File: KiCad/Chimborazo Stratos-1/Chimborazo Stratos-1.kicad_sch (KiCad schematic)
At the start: 0 parts

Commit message: fixed long path errors and cleaned up libraries, finally I added the libs for the project it was REALLY HARD AND I DONT KNOW WHY :( but I managed to overcome the challenge
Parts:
- added U1: RP2040, Package_DFN_QFN:QFN-56-1EP_7x7mm_P0.4mm_EP3.2x3.2mm, symbol MCU_RaspberryPi:RP2040
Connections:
- new net: U1.1 (IOVDD), U1.10 (IOVDD), U1.22 (IOVDD), U1.33 (IOVDD), U1.42 (IOVDD), U1.49 (IOVDD)
- new net: U1.23 (DVDD), U1.50 (DVDD)
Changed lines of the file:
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@@
 	(generator_version "9.0")
 	(paper "A4")
+	(symbol
+		(lib_id "MCU_RaspberryPi:RP2040")
+		(at 140.97 80.01 0)
+		(unit 1)
+		(exclude_from_sim no)
+		(in_bom yes)
+		(on_board yes)
+		(dnp no)
+		(fields_autoplaced yes)
+		(property "Reference" "U1"
+			(at 143.1133 124.46 0)
+			(effects
+				(font
+					(size 1.27 1.27)
+				)
+				(justify left)
+			)
+		)
+		(property "Value" "RP2040"
+			(at 143.1133 127 0)
+			(effects
+				(font
+					(size 1.27 1.27)
+				)
+				(justify left)
+			)
+		)
+		(property "Footprint" "Package_DFN_QFN:QFN-56-1EP_7x7mm_P0.4mm_EP3.2x3.2mm"
+			(at 140.97 80.01 0)
+			(effects
+				(font
+					(size 1.27 1.27)
+				)
+				(hide yes)
+			)
+		)
+		(property "Datasheet" "https://datasheets.raspberrypi.com/rp2040/rp2040-datasheet.pdf"
+			(at 140.97 80.01 0)
+			(effects
+				(font
+					(size 1.27 1.27)
+				)
+				(hide yes)
+			)
+		)
+		(property "Description" "A microcontroller by Raspberry Pi"
+			(at 140.97 80.01 0)
+			(effects
+				(font
+					(size 1.27 1.27)
+				)
+				(hide yes)
+			)
+		)
+		(pin "13"
+		)
+		(pin "27"
+		)
+		(pin "20"
+		)
+		(pin "48"
+		)
+		(pin "46"
+		)
+		(pin "55"
+		)
+		(pin "34"
+		)
+		(pin "36"
+		)
+		(pin "38"
+		)
+		(pin "40"
+		)
+		(pin "19"
+		)
+		(pin "56"
+		)
+		(pin "15"
+		)
+		(pin "54"
+		)
+		(pin "10"
+		)
+		(pin "45"
+		)
+		(pin "53"
+		)
+		(pin "42"
+		)
+		(pin "26"
+		)
+		(pin "4"
+		)
+		(pin "47"
+		)
+		(pin "57"
+		)
+		(pin "5"
+		)
+		(pin "51"
+		)
+		(pin "43"
+		)
+		(pin "3"
+		)
+		(pin "33"
+		)
+		(pin "1"
+		)
+		(pin "50"
+		)
+		(pin "2"
+		)
+		(pin "6"
+		)
+		(pin "7"
+		)
+		(pin "9"
+		)
+		(pin "11"
+		)
+		(pin "21"
+		)
+		(pin "8"
+		)
+		(pin "12"
+		)
+		(pin "24"
+		)
+		(pin "25"
+		)
+		(pin "23"
+		)
+		(pin "52"
+		)
+		(pin "49"
+		)
+		(pin "44"
+		)
+		(pin "14"
+		)
+		(pin "22"
+		)
+		(pin "16"
+		)
+		(pin "17"
+		)
+		(pin "18"
+		)
+		(pin "28"
+		)
+		(pin "29"
+		)
+		(pin "30"
+		)
+		(pin "31"
+		)
+		(pin "32"
+		)
+		(pin "35"
+		)
+		(pin "37"
+		)
+		(pin "39"
+		)
+		(pin "41"
+		)
+		(instances
+			(project ""
+				(path "/693bdab5-43ca-4fa8-b8fd-c6e41a7a7cc1"
+					(reference "U1")
+					(unit 1)
+				)
+			)
+		)
+	)
 	(sheet_instances
 		(path "/"

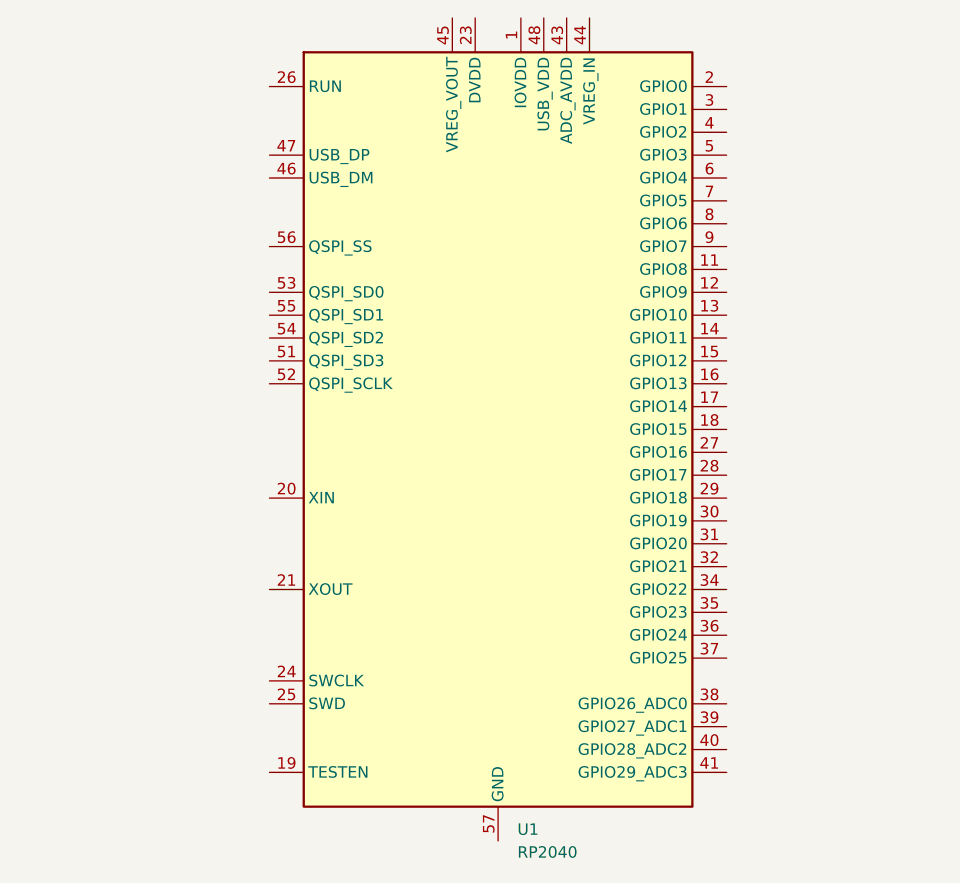
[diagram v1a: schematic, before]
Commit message: Schematic prototype done
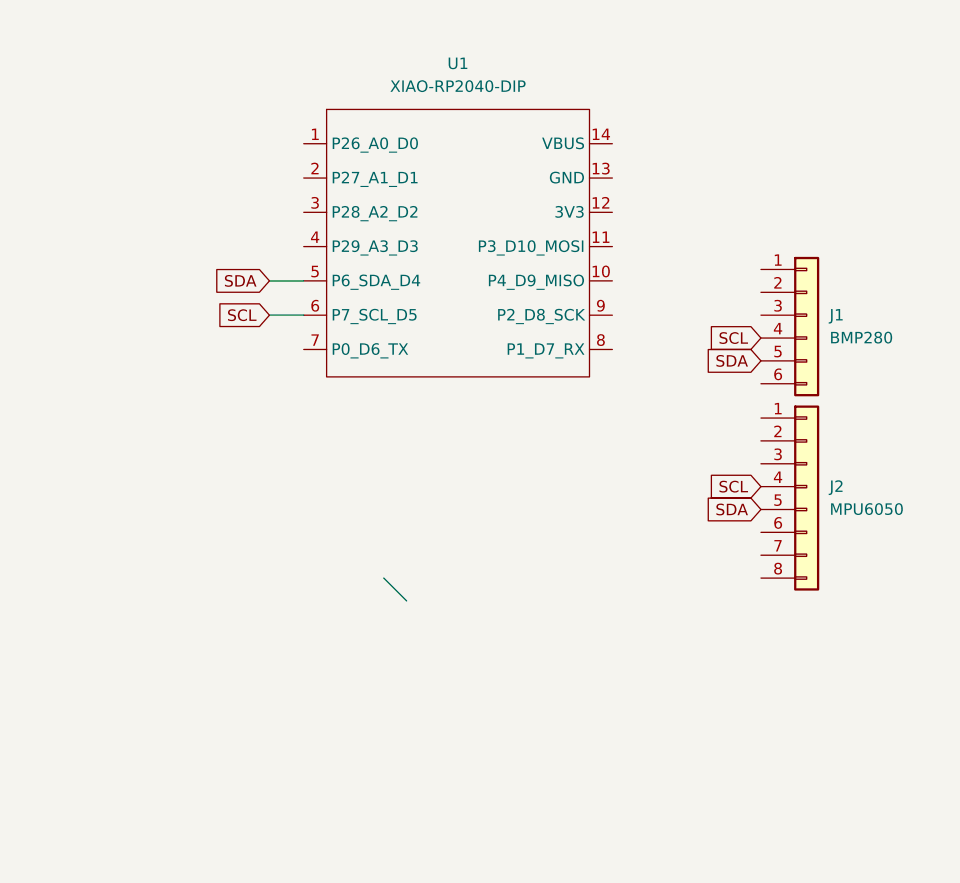
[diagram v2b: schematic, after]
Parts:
- removed U1: RP2040, Package_DFN_QFN:QFN-56-1EP_7x7mm_P0.4mm_EP3.2x3.2mm, symbol MCU_RaspberryPi:RP2040
- added J1: BMP280, symbol Connector_Generic:Conn_01x06
- added J2: MPU6050, symbol Connector_Generic:Conn_01x08
- added U1: XIAO-RP2040-DIP, Seeed_Studio_XIAO_Series:XIAO-RP2040-DIP, symbol Seeed_Studio_XIAO_Series:XIAO-RP2040-DIP
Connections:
- new net SCL: J1.4 (Pin_4), J2.4 (Pin_4), U1.6 (P7_SCL_D5)
- new net SDA: J1.5 (Pin_5), J2.5 (Pin_5), U1.5 (P6_SDA_D4)

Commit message: PCB model 1 finalized
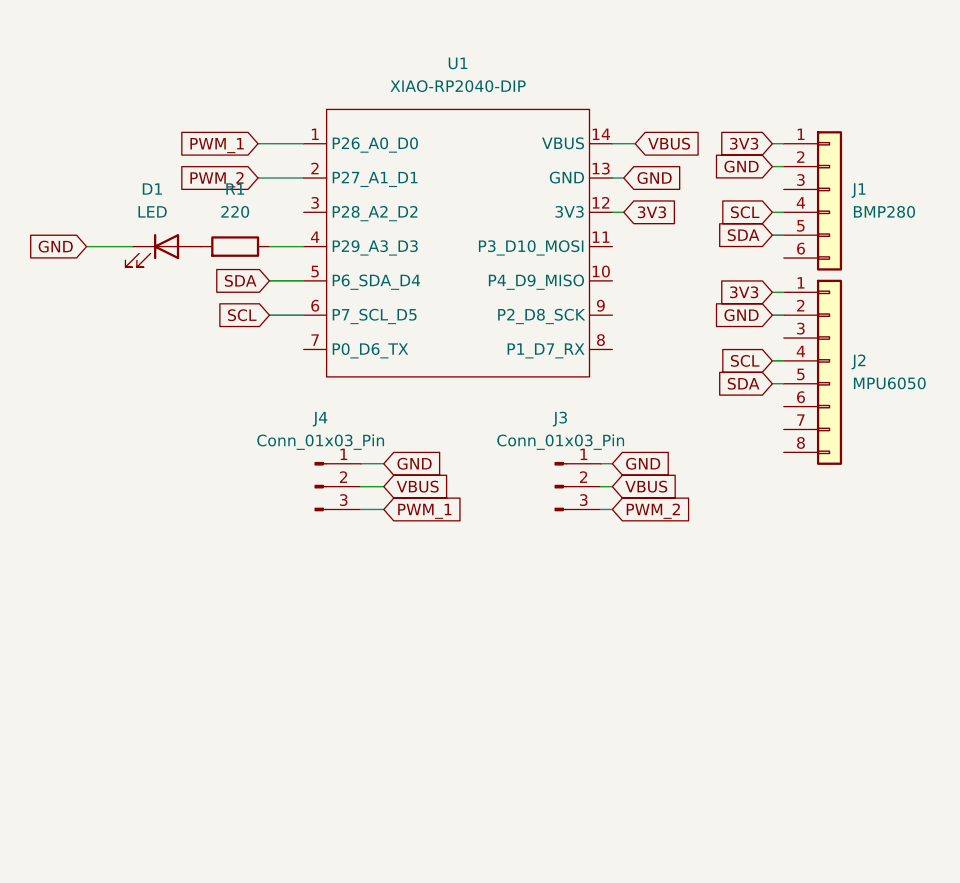
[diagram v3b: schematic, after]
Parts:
- added D1: LED, LED_THT:LED_D5.0mm, symbol Device:LED
- added J3, J4: Conn_01x03_Pin, Connector:FanPinHeader_1x03_P2.54mm_Vertical, symbol Connector:Conn_01x03_Pin
- added R1: 220, Resistor_THT:R_Axial_DIN0207_L6.3mm_D2.5mm_P7.62mm_Horizontal, symbol Device:R
- J1: footprint (none) -> Connector_PinHeader_2.54mm:PinHeader_1x06_P2.54mm_Vertical
- J2: footprint (none) -> Connector_PinHeader_2.54mm:PinHeader_1x08_P2.54mm_Vertical
- U1: footprint Seeed_Studio_XIAO_Series:XIAO-RP2040-DIP -> Seeed Studio XIAO Series Library:XIAO-RP2040-DIP
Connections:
- net PWM_1: now reaches U1.1 (P26_A0_D0)
- net PWM_1: now also J4.3 (Pin_3)
- net 3V3: now reaches U1.12 (3V3)
- net 3V3: now also J1.1 (Pin_1), J2.1 (Pin_1)
- net GND: now reaches U1.13 (GND)
- net GND: now also J1.2 (Pin_2), J2.2 (Pin_2), D1.1 (K), J3.1 (Pin_1), J4.1 (Pin_1)
- net VBUS: now reaches U1.14 (VBUS)
- net VBUS: now also J3.2 (Pin_2), J4.2 (Pin_2)
- net PWM_2: now reaches U1.2 (P27_A1_D1)
- net PWM_2: now also J3.3 (Pin_3)
- net at U1.4 (P29_A3_D3): now also R1.1
- new net: D1.2 (A), R1.2
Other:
- moved on the sheet: J1, J2
